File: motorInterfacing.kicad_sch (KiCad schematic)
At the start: 4 parts, among them J1 Conn_01x02, J2 Conn_01x02_Socket

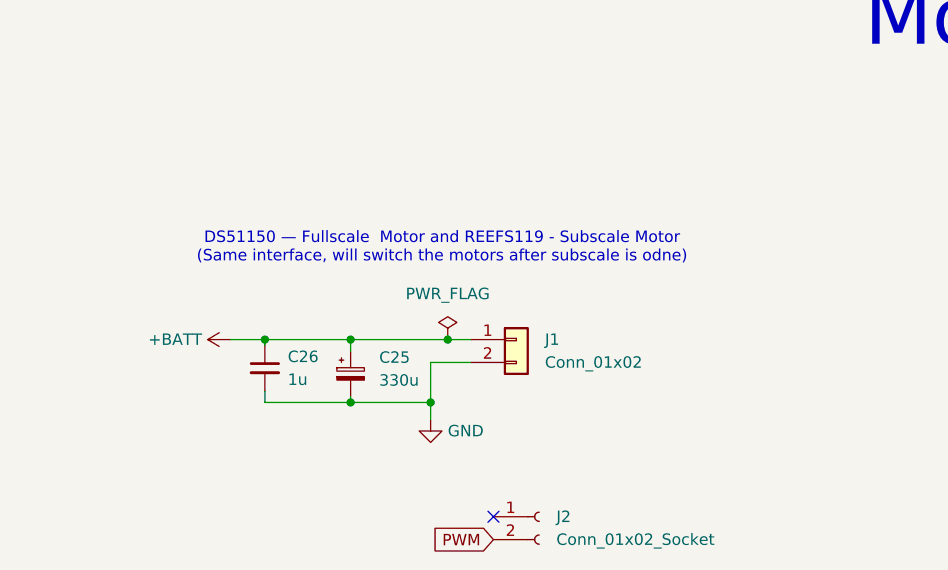
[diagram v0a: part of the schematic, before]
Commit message: finalized
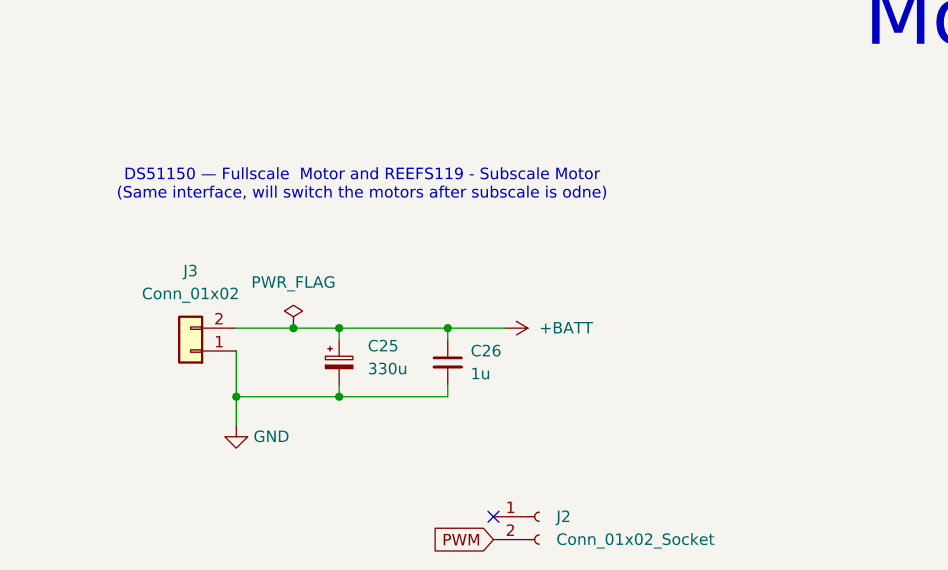
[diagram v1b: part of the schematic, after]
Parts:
- removed J1: Conn_01x02, Connector_AMASS:AMASS_XT30U-F_1x02_P5.0mm_Vertical, symbol Connector_Generic:Conn_01x02
- added J3: Conn_01x02, Connector_AMASS:AMASS_XT30U-F_1x02_P5.0mm_Vertical, symbol Connector_Generic:Conn_01x02
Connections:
- net +BATT: now also J3.2 (Pin_2)
- net GND: now also J3.1 (Pin_1)
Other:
- moved on the sheet: C26
